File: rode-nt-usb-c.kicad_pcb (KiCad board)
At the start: 2 copper layers, 36 x 15 mm, 5 parts, among them J1 USB_C_Receptacle, J2 Conn_01x05_Pin

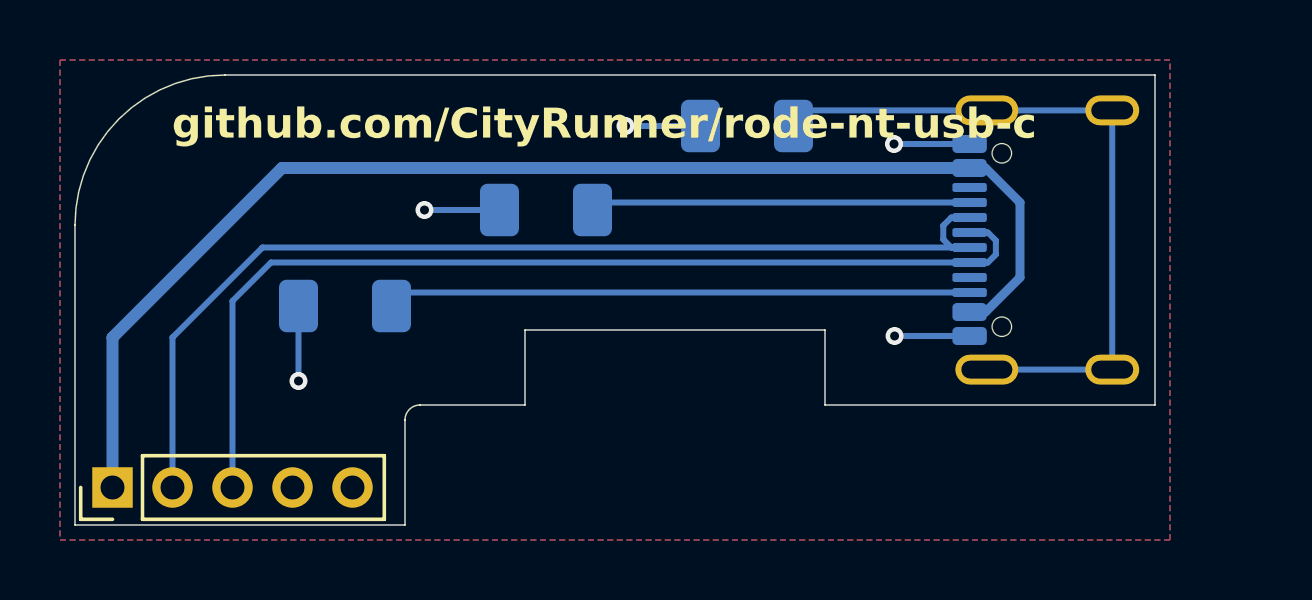
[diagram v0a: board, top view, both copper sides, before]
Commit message: Change cutouts
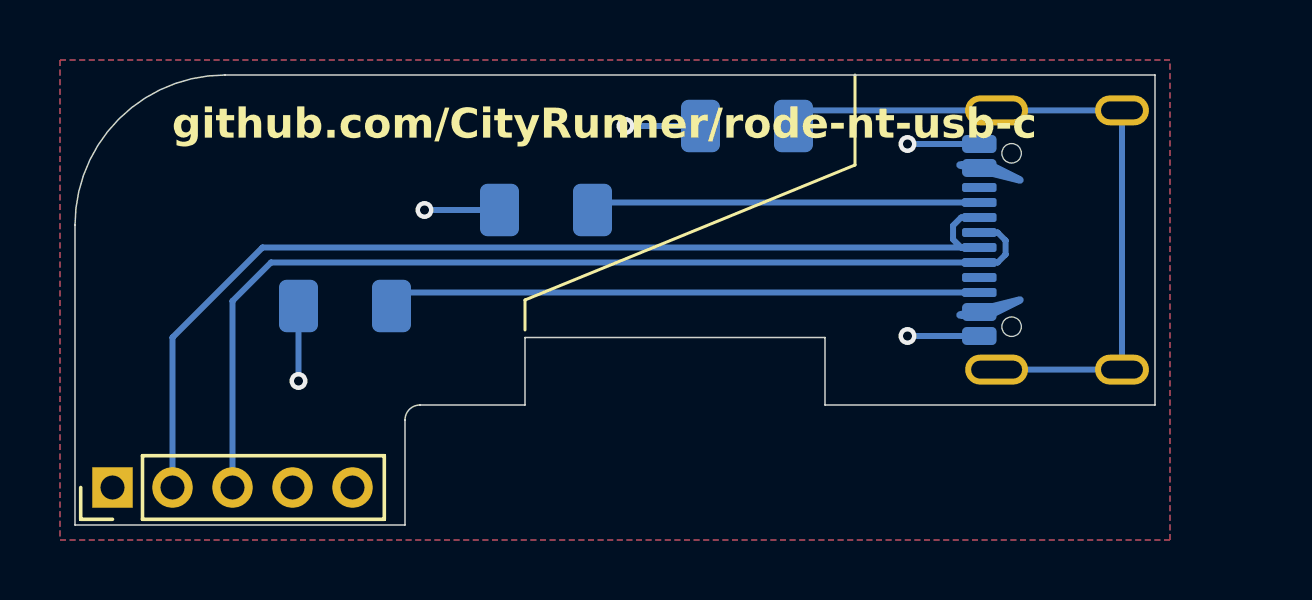
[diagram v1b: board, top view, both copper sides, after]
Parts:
- moved J1 0.33 mm to (109.8, 59.0)
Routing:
- net +5V: track 43.3 -> 0.00 mm
- added copper zone on B.Cu, net +5V
- removed copper zone on B.Cu, net (none)
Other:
- outline, holes or cut-outs redrawn
